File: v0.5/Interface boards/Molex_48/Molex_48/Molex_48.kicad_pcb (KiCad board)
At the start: 2 copper layers, 2 parts, among them J1 Conn_02x20_Counter_Clockwise, J2 500762-0482

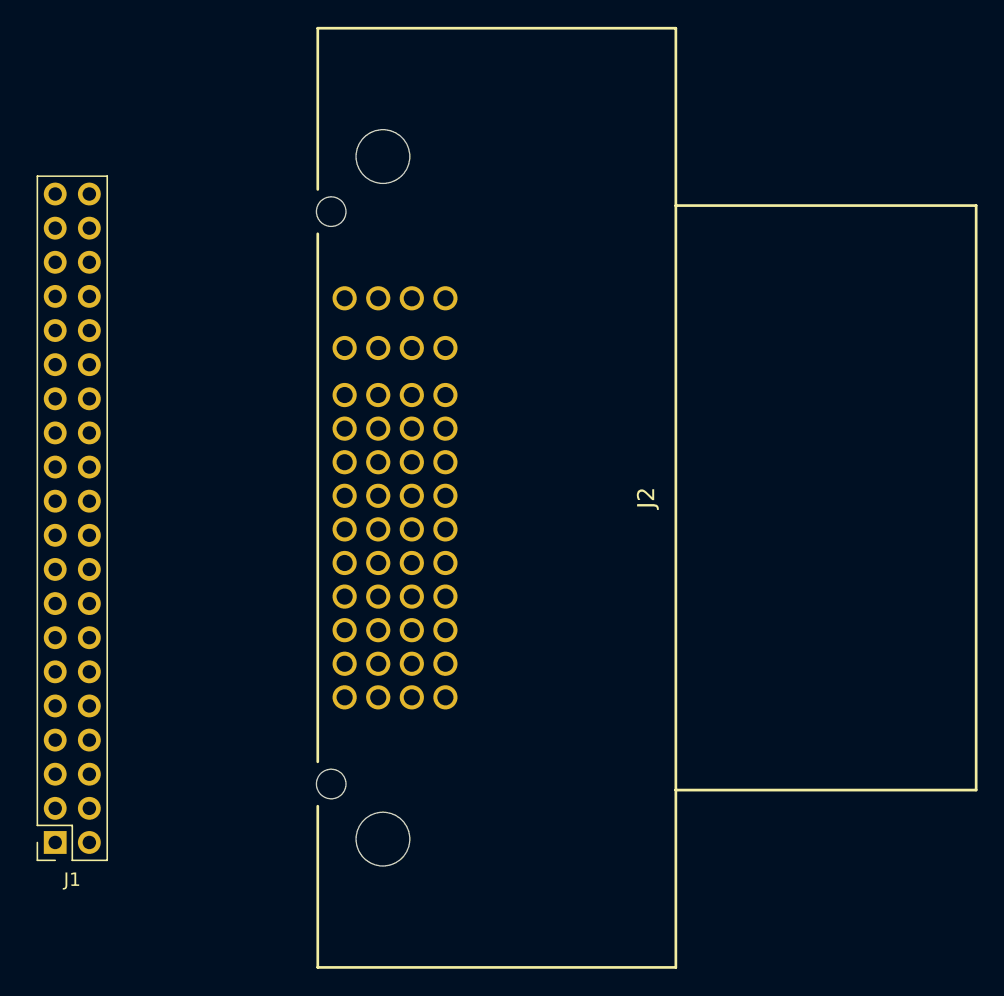
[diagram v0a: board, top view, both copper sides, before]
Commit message: update
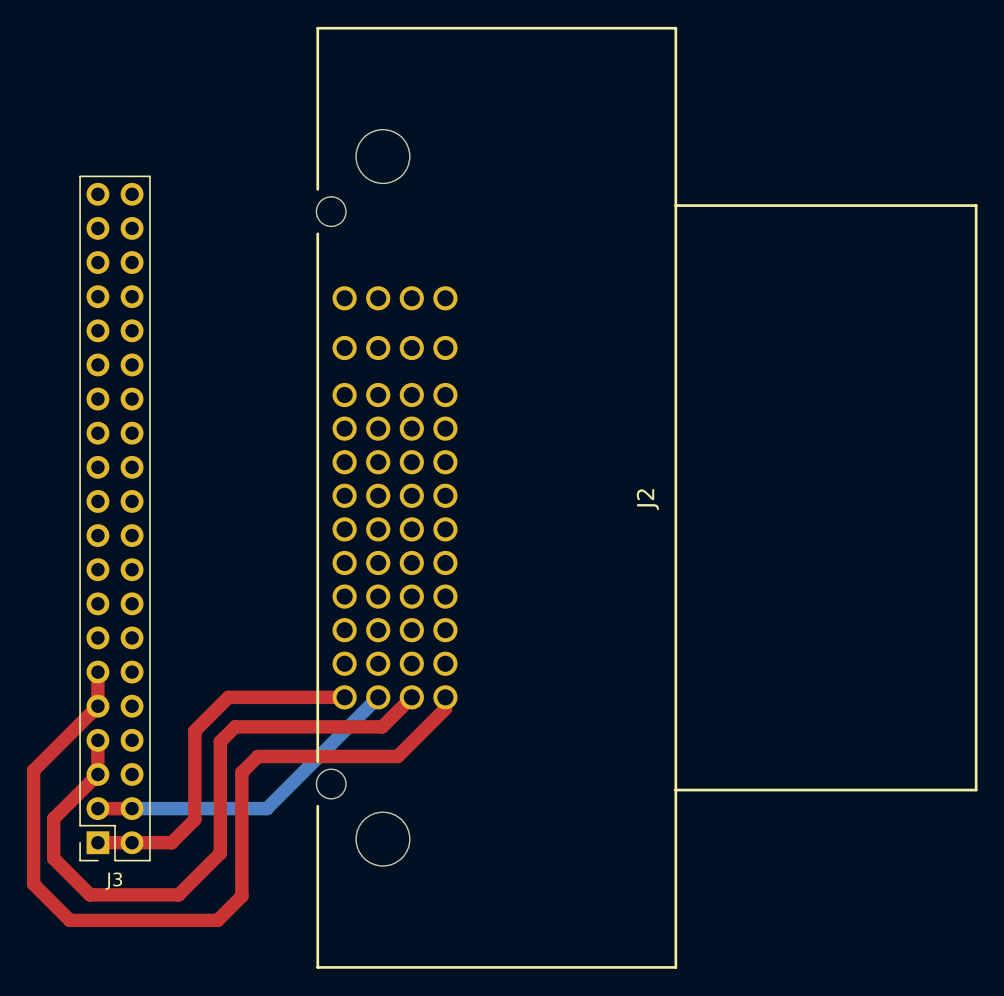
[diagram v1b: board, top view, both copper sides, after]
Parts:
- removed J1: Conn_02x20_Counter_Clockwise, Connector_PinSocket_2.54mm:PinSocket_2x20_P2.54mm_Vertical
- added J3: Conn_02x20_Odd_Even, Connector_PinSocket_2.54mm:PinSocket_2x20_P2.54mm_Vertical, F.Cu at (105.4, 120.6)
- J2: footprint SamacSys_Parts:5007620482 -> libs:5007620482
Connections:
- J2 pad A1: Injector_1_-_Pin_1-2 -> Injector_1
- J2 pad A2: Injector_2_-_Pin_1-2 -> Injector_2
- J2 pad A3: Injector_3_-_Pin_1-2 -> Injector_3
- J2 pad A4: Injector_4_-_Pin_1-2 -> Injector_4
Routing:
- net Injector_4: track 0.00 -> 62.3 mm
- net Injector_3: track 0.00 -> 48.9 mm
- net Injector_1: track 0.00 -> 26.7 mm
- net Injector_2: track 0.00 -> 24.3 mm
